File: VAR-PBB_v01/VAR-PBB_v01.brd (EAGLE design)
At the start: 78.4 x 86.4 mm, 20 parts, among them J1 ANDERSON_POWER_POLE, J11 CON1X2_SHROUDED, J2 ANDERSON_POWER_POLE, J3 CON1X2_SHROUDED, J4 CON1X2_SHROUDED, J5 CON1X2_SHROUDED, J6 CON1X2_SHROUDED, J7 CON1X2_SHROUDED, J8 CON1X2_SHROUDED, U1 OKI-78SR, U2 XL6009, U3 XL6009, U4 XL6009

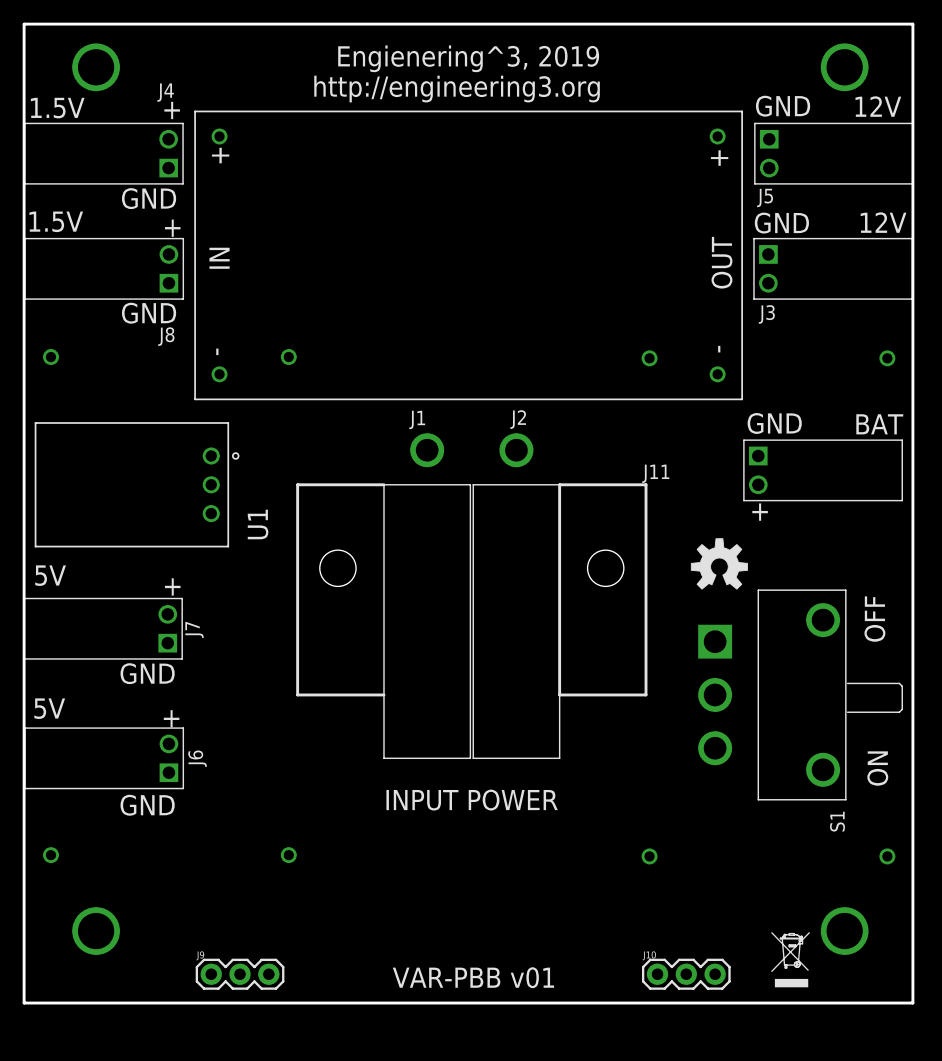
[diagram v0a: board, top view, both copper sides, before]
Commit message: WIP, but got a ton done.
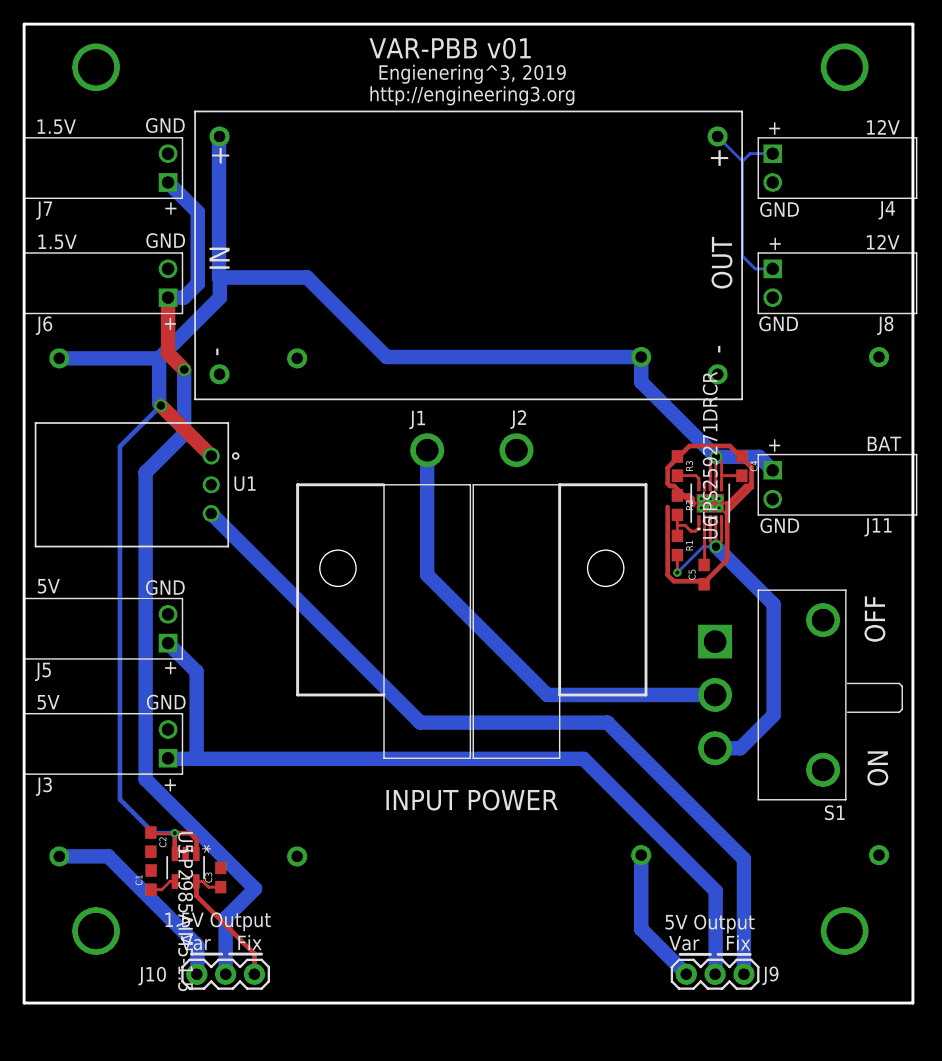
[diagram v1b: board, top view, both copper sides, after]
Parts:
- added C1, C4, C5: 0.1uF, SparkFun-Capacitors:0603
- added C2: 1.0uF, SparkFun-Capacitors:0603
- added C3: 2.2uF, SparkFun-Capacitors:0603
- added R1, R2, R3: (no value), SparkFun-Resistors:0603
- added U5: LP2985AIM5-1.5, LP2985AIM5-1.5:MF05A
- added U6: TPS259271DRCR, TPS259271DRCR:DRC10_1P65X2P40
- moved U$5 91.8 mm to (18.6, 80.0), flipped to the bottom
- moved J5 67.6 mm to (12.7, 33.0), turned to 0 degrees
- moved J3 67.5 mm to (12.7, 22.9), turned to 0 degrees
- moved J4 53.3 mm to (66.0, 73.7), turned to 180 degrees
- moved J8 53.3 mm to (66.0, 63.5), turned to 180 degrees
- moved U3 52.1 mm to (64.9, 35.0)
- moved U4 52.1 mm to (13.6, 34.9)
- moved J9 47.0 mm to (63.5, 2.54), turned to 180 degrees
- moved LOGO1 44.0 mm to (59.1, 82.4), flipped to the bottom
- moved J6 41.9 mm to (12.7, 63.5)
- moved J7 40.6 mm to (12.7, 73.7)
- moved J10 35.6 mm to (20.3, 2.54), turned to 180 degrees
- moved J11 1.80 mm to (66.0, 45.7)
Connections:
- removed net N$6: J10.1
- new net 1.5V_REG: C3.1, J10.1, U5.5
- new net N$12: R3.2, U6.10
- new net N$13: C5.2, U6.2
- new net N$14: R1.1, R2.2, U6.1
- new net N$8: C1.1, U5.4
- net BATT+: now also C2.1, C4.2, U5.1, U5.3, U6.6, U6.7, U6.8
- net GND: now also C1.2, C2.2, C3.2, C4.1, C5.1, R2.1, R3.1, U5.2, U6.11
- net N$1: now also R1.2, U6.3, U6.4, U6.5
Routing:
- net BATT+: track 0.00 -> 158.1 mm, vias 0 -> 3
- net CHANNEL4: track 0.00 -> 79.9 mm, vias 0 -> 1
- net CHANNEL3: track 0.00 -> 71.8 mm
- net 5V_REG: track 0.00 -> 69.8 mm
- net N$11: track 0.00 -> 40.8 mm
- net GND: track 0.00 -> 40.7 mm, vias 0 -> 4
- net N$1: track 0.00 -> 36.7 mm, vias 0 -> 2
- net N$7: track 0.00 -> 18.0 mm
- net N$5: track 0.00 -> 17.5 mm
- net 1.5V_REG: track 0.00 -> 12.6 mm
- net N$3: track 0.00 -> 12.2 mm
- net N$14: track 0.00 -> 4.78 mm
- net N$13: track 0.00 -> 3.99 mm
- net N$12: track 0.00 -> 2.71 mm
- net N$8: track 0.00 -> 2.39 mm
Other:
- board text added: "1.5V Output"
- board text added: "5V Output"
- board text added: "Fix"
- board text added: "Var"
